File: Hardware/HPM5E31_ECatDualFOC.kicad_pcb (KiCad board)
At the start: 4 copper layers, 85 x 113.4 mm, 576 parts, among them J1 Conn_Coaxial, J13 PHB2.0-02-20PWZ, J14 PHB2.0-02-20PWZ, J15 RJ45_Hanrun_HR911105A_Horizon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, J16 RJ45_Hanrun_HR911105A_Horizon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, J17 WAFER-GH1.25-4PWB, J18 WAFER-GH1.25-4PWB, J19 WAFER-GH1.25-4PWB, J2 Conn_Coaxial, J20 WAFER-GH1.25-2PWB, J21 WAFER-GH1.25-2PWB, J22 USB_B, J23 WAFER-GH1.25-4PWB, J24 WAFER-GH1.25-4PLB, J3 WAFER-ZH1.5-4PWB, J4 Conn_02x05_Odd_Even, J5 WAFER-GH1.25-6PWB, J6 Conn_02x05_Odd_Even, K1 DSHP02TSGET, Q1 CSD19532Q5B, Q10 CSD19532Q5B, Q11 CSD19532Q5B, Q12 CSD19532Q5B, Q13 CSD19532Q5B, Q14 NCE01ND03S, Q15 CSD19532Q5B, Q16 NCE01ND03S, Q2 CSD19532Q5B, Q3 CSD19532Q5B, Q4 CSD19532Q5B, Q5 CSD19532Q5B, Q6 CSD19532Q5B, Q7 CSD19532Q5B, Q8 CSD19532Q5B, Q9 CSD19532Q5B, U1 TXS0108ERGYR, U10 REF3030AIDBZR, U11 MX25L12833FM2I-10G, U12 UCC27282DRCR, U13 INA240A1PWR, U14 UCC27282DRCR, U15 INA240A1PWR, U16 UCC27282DRCR, U17 INA240A1PWR, U18 74LVC1G08, U19 INA240A1PWR, U2 TXB0104RUTR, U20 UCC27282DRCR, U21 INA240A1PWR, U22 UCC27282DRCR, U23 INA240A1PWR, U24 UCC27282DRCR, U25 INA240A1PWR, U26 74LVC1G08, U27 INA240A1PWR, U28 PY32F002BF15U, U29 EG2104, U3 HPM5E31IGN1, U30 ZX-HY2.0-2PWT, U31 RT9193-33GB-MS, U32 EG2104, U33 ZX-HY2.0-2PWT, U34 M3, U35 RS622XTDE8, U36 74LVC1G08, U37 74LVC1G08, U38 M3, U39 MS2575T, U4 LM5164DDAR, U40 MS2575T, U41 TXB0104RUTR, U42 MS2575T, U43 MS2575T, U44 TXB0104RUTR, U45 JL1111-N032I, U46 M3, U47 M3, U48 JL1111-N032I, U49 SP3485EN-L/TR, U5 MP1605GTF-Z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

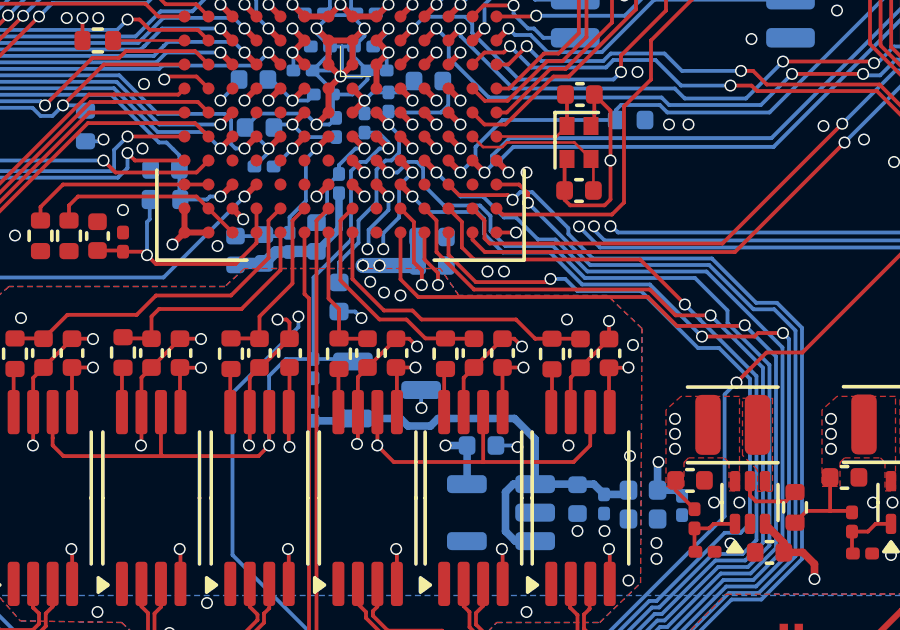
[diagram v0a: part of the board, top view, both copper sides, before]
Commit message: Update HPM5E31_ECatDualFOC.kicad_pcb
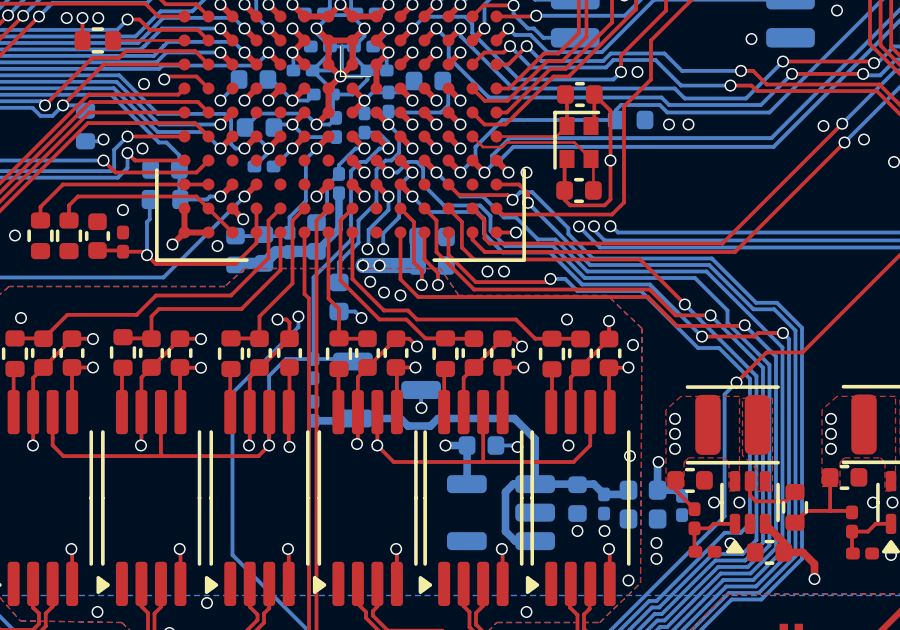
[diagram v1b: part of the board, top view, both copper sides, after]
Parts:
- R96, R97: value 2R,1% -> 5.1R,1%
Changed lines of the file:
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@@
 			)
 		)
-		(property "Value" "2R,1%"
+		(property "Value" "5.1R,1%"
 			(at 0 -1.17 0)
 			(layer "B.Fab")
@@
 			)
 		)
-		(property "Description" "2Ω ±1% 62.5mW 厚膜电阻"
+		(property "Description" "5.1Ω ±1% 62.5mW 厚膜电阻"
 			(at 0 0 0)
 			(layer "B.Fab")
@@
 			)
 		)
-		(property "立创编号" "C270630"
+		(property "立创编号" "C25128"
 			(at 0 0 0)
 			(unlocked yes)
@@
 			)
 		)
-		(property "Value" "2R,1%"
+		(property "Value" "5.1R,1%"
 			(at 0 -1.17 0)
 			(layer "B.Fab")
@@
 			)
 		)
-		(property "Description" "2Ω ±1% 62.5mW 厚膜电阻"
+		(property "Description" "5.1Ω ±1% 62.5mW 厚膜电阻"
 			(at 0 0 0)
 			(layer "B.Fab")
@@
 			)
 		)
-		(property "立创编号" "C270630"
+		(property "立创编号" "C25128"
 			(at 0 0 0)
 			(unlocked yes)
@@
 	)
 	(segment
-		(start 105.4966 109.8034)
-		(end 105.4966 111.3466)
+		(start 113.09 113.34)
+		(end 113.1 113.35)
 		(width 0.127)
 		(layer "F.Cu")
@@
 	)
 	(segment
-		(start 105.5 109.8)
-		(end 105.4966 109.8034)
+		(start 106.55 112.4)
+		(end 107.35 112.4)
 		(width 0.127)
 		(layer "F.Cu")
@@
 	)
 	(segment
-		(start 111.59 113.34)
-		(end 112.15 113.34)
+		(start 105.4966 111.3466)
+		(end 106.55 112.4)
 		(width 0.127)
 		(layer "F.Cu")
@@
 	)
 	(segment
-		(start 105.4966 111.3466)
-		(end 106.55 112.4)
+		(start 107.65 112.7)
+		(end 110.95 112.7)
 		(width 0.127)
 		(layer "F.Cu")
@@
 	)
 	(segment
-		(start 107.5 112.4)
-		(end 107.8 112.7)
+		(start 110.95 112.7)
+		(end 111.59 113.34)
 		(width 0.127)
 		(layer "F.Cu")
@@
 	)
 	(segment
-		(start 106.55 112.4)
-		(end 107.5 112.4)
+		(start 105.5 109.8)
+		(end 105.4966 109.8034)
 		(width 0.127)
 		(layer "F.Cu")
@@
 	)
 	(segment
-		(start 113.09 113.34)
-		(end 113.1 113.35)
+		(start 111.59 113.34)
+		(end 112.15 113.34)
 		(width 0.127)
 		(layer "F.Cu")
@@
 	)
 	(segment
-		(start 110.95 112.7)
-		(end 111.59 113.34)
+		(start 105.4966 109.8034)
+		(end 105.4966 111.3466)
 		(width 0.127)
 		(layer "F.Cu")
@@
 	)
 	(segment
-		(start 107.8 112.7)
-		(end 110.95 112.7)
+		(start 107.35 112.4)
+		(end 107.65 112.7)
 		(width 0.127)
 		(layer "F.Cu")
